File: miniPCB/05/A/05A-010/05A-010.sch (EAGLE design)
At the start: 6 parts

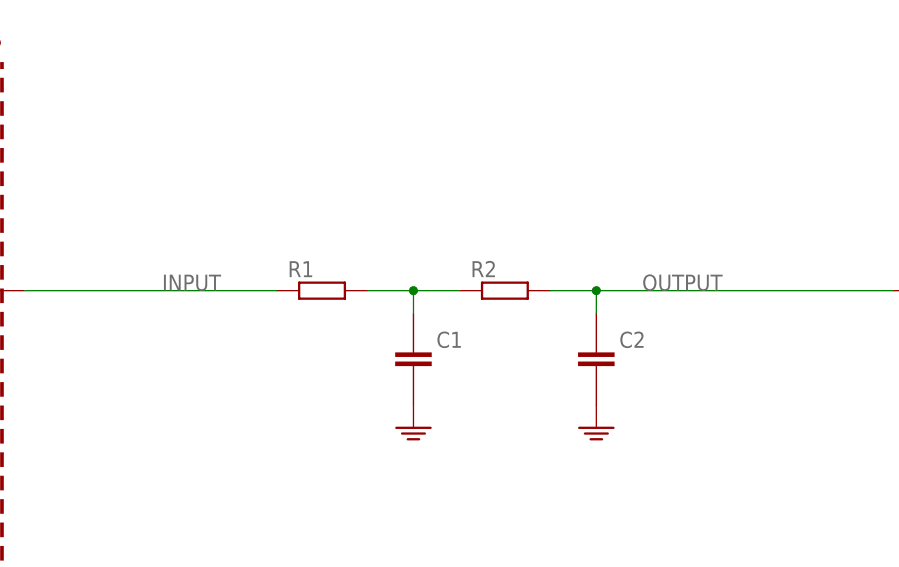
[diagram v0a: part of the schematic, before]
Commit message: Attempting to fix my Git merge error.
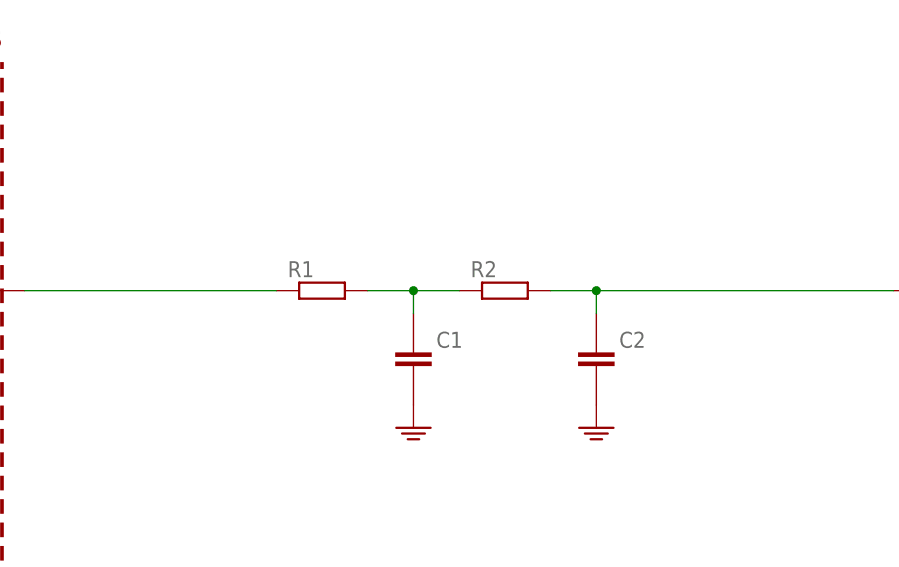
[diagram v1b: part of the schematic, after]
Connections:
- net INPUT renamed N$1
- net OUTPUT renamed N$3
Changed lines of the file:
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@@
 <layer number="96" name="Values" color="7" fill="1" visible="yes" active="yes"/>
 <layer number="97" name="Info" color="7" fill="1" visible="yes" active="yes"/>
-<layer number="98" name="Guide" color="6" fill="1" visible="no" active="yes"/>
+<layer number="98" name="Guide" color="6" fill="1" visible="yes" active="yes"/>
 <layer number="99" name="SpiceOrder" color="7" fill="1" visible="no" active="no"/>
 <layer number="100" name="Muster" color="7" fill="1" visible="no" active="no"/>
@@
 </segment>
 </net>
-<net name="INPUT" class="0">
+<net name="N$1" class="0">
 <segment>
 <pinref part="P1" gate="-4" pin="1"/>
 <pinref part="R1" gate="R" pin="1"/>
 <wire x1="43.18" y1="116.84" x2="71.12" y2="116.84" width="0.1524" layer="91"/>
-<label x="58.42" y="116.84" size="1.778" layer="95"/>
 </segment>
 </net>
@@
 </segment>
 </net>
-<net name="OUTPUT" class="0">
+<net name="N$3" class="0">
 <segment>
 <pinref part="R2" gate="R" pin="2"/>
@@
 <wire x1="106.68" y1="116.84" x2="139.7" y2="116.84" width="0.1524" layer="91"/>
 <junction x="106.68" y="116.84"/>
-<label x="111.76" y="116.84" size="1.778" layer="95"/>
-</segment>
-</net>
+</segment>
+</net>
